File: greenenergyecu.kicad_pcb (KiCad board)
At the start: 4 copper layers, 164 x 118 mm, 103 parts, among them J21 Conn_01x05_Male, J22 USB_B_Mini, M1 Module-power_12and5V-0.3, M2 Module-knock-0.2, M3 Module-vr-discrete-0.5, M4 Module-vr-max9924-0.1, M5 Module-wbo-0.5, M6 Module:mega-mcu100/0.3, M7 Module-can-0.1, M8 Module-motor-driver-0.1, P1 368255-2, Q1 ISL9V3040D3ST, Q2 ISL9V3040D3ST, Q3 ISL9V3040D3ST, Q4 ISL9V3040D3ST, Q5 ISL9V3040D3ST, Q6 ISL9V3040D3ST, Q7 AO3400A, U1 VNLD5160TR-E, U10 BTS6143D, U2 VNLD5160TR-E, U3 VNLD5160TR-E, U4 VNLD5160TR-E, U5 VNLD5160TR-E, U6 VNLD5160TR-E, U7 VNLD5160TR-E, U8 MAX31855KASA

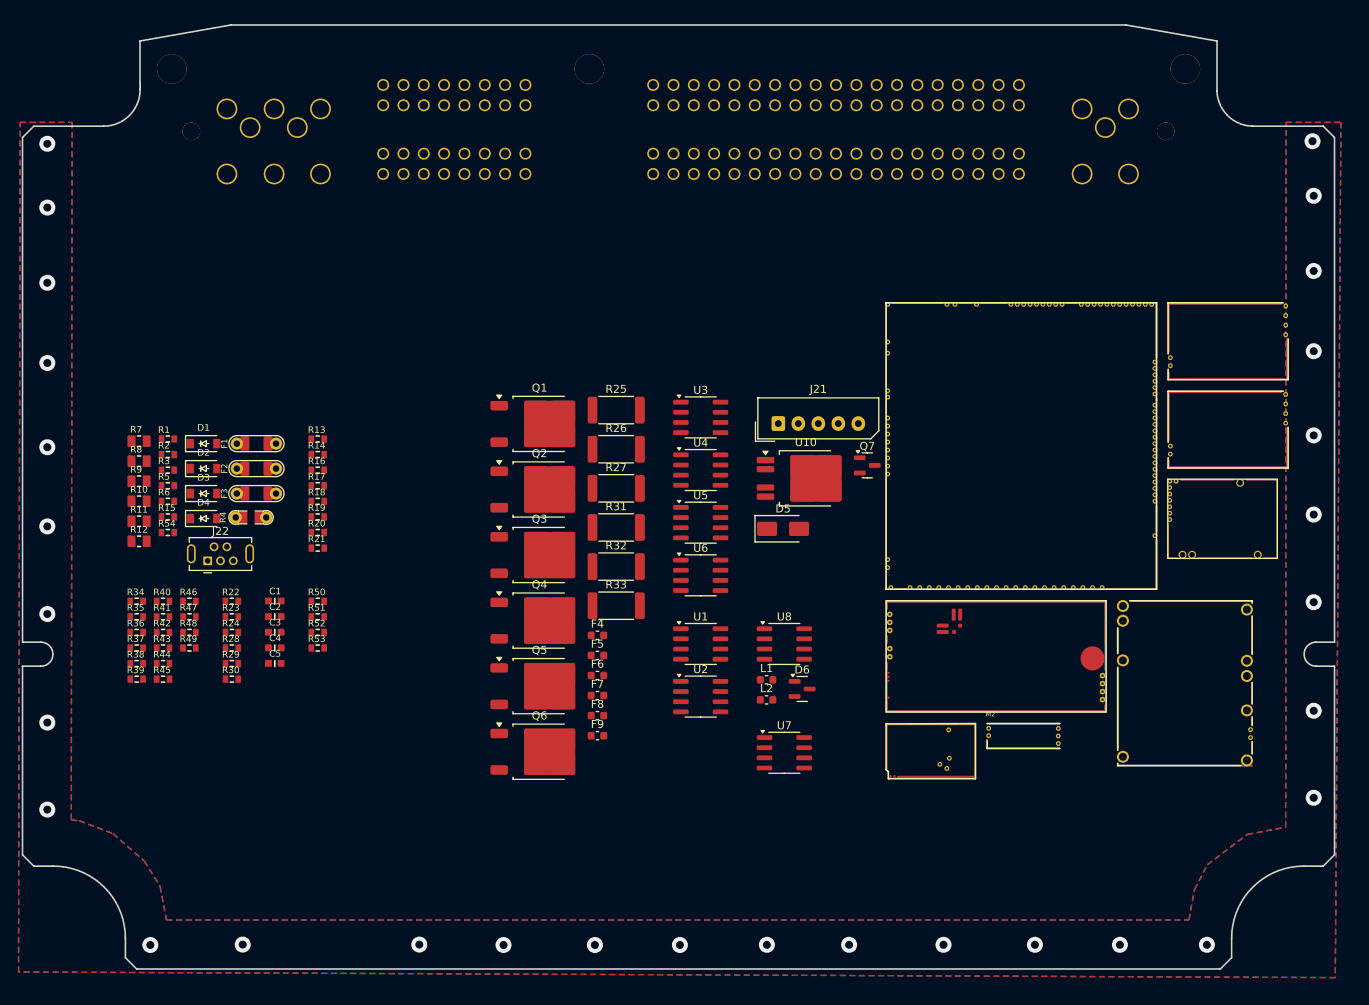
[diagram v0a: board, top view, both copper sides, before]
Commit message: weW
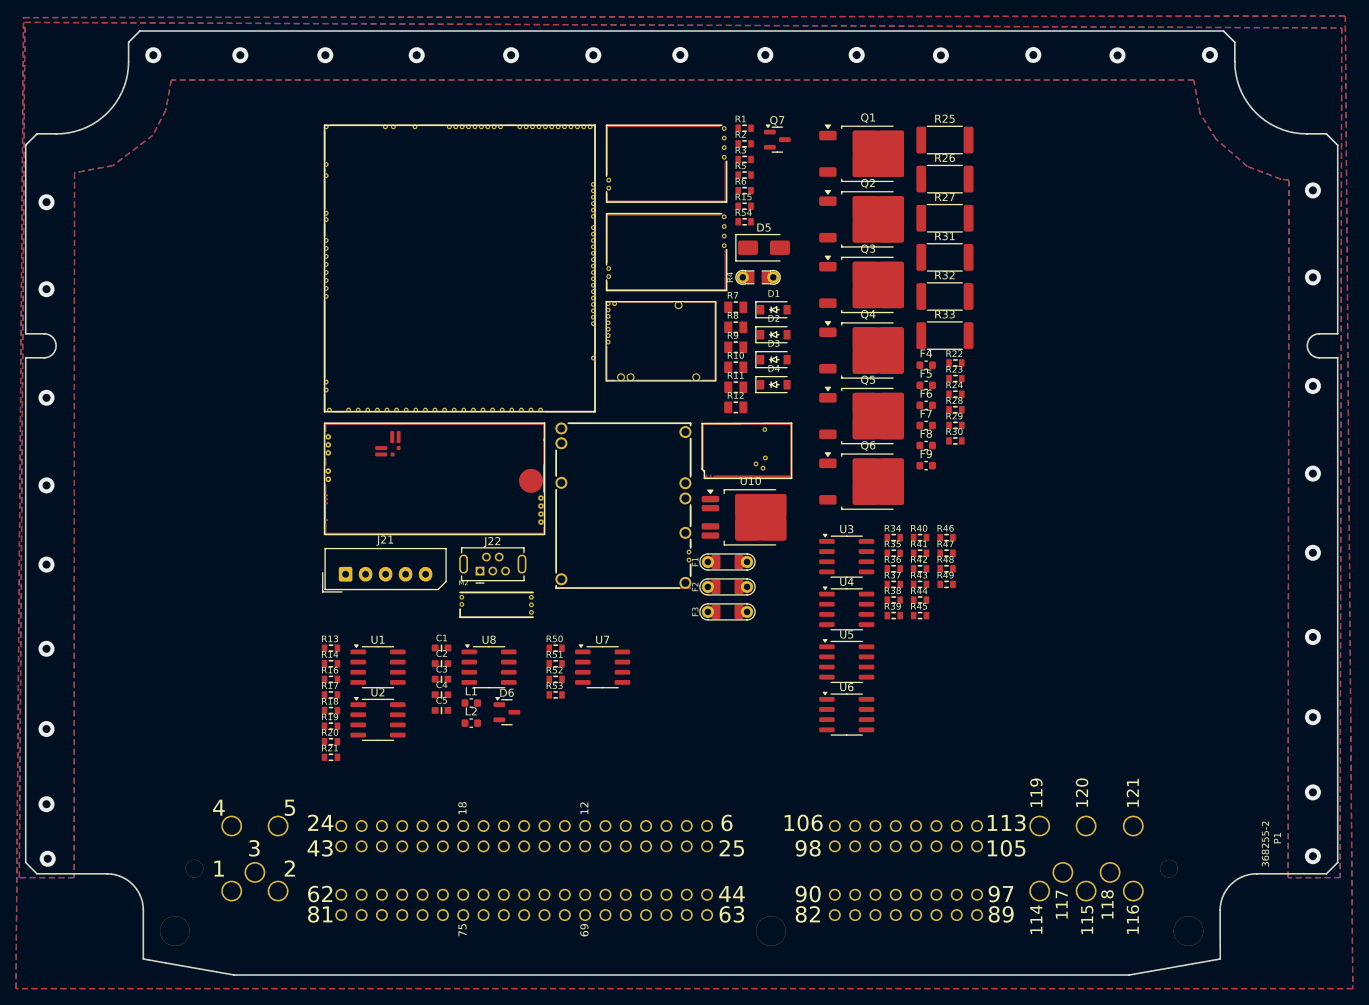
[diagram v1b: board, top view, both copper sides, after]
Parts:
- added G4: DISCLAIMER, rusefi_lib:Off_Road_Disclaimer, B.Cu at (111.8, 0.28)
- P1: footprint 368255-2:368255-2 -> hellen121vag:368255-2
- moved P1 139.4 mm to (60.2, 32.9), turned to 0 degrees
- moved R22 95.2 mm to (161.9, 33.9)
- moved R23 95.2 mm to (161.9, 35.8)
- moved R24 95.2 mm to (161.9, 37.8)
- moved R28 95.2 mm to (161.9, 39.7)
- moved R29 95.2 mm to (161.9, 41.7)
- moved R30 95.2 mm to (161.9, 43.6)
- moved R46 95.0 mm to (160.8, 55.7)
- moved R47 95.0 mm to (160.8, 57.7)
- moved R48 95.0 mm to (160.8, 59.6)
- moved R49 95.0 mm to (160.8, 61.6)
- moved R34 95.0 mm to (154.2, 55.7)
- moved R35 95.0 mm to (154.2, 57.7)
- moved R36 95.0 mm to (154.2, 59.6)
- moved R37 95.0 mm to (154.2, 61.6)
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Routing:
- net PIN2: vias 0 -> 31
- net PIN113: vias 30 -> 0
- added copper zone on B.Cu, net PIN2
- added copper zone on F.Cu, net PIN2
- added copper zone on In1.Cu, net PIN2
- removed copper zone on B.Cu, net PIN113
- removed copper zone on F.Cu, net PIN113
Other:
- outline, holes or cut-outs redrawn
- board text added: "1"
- board text added: "10"
- board text added: "100"
- board text added: "101"
- board text added: "102"
- board text added: "103"
- board text added: "104"
- board text added: "105"
- board text added: "106"
- board text added: "11"
- board text added: "112"
- board text added: "113"
- board text added: "114"
- board text added: "115"
- board text added: "116"
- board text added: "117"
- board text added: "118"
- board text added: "119"
- board text added: "12"
- board text added: "120"
- board text added: "121"
- board text added: "13"
- board text added: "14"
- board text added: "15"
- board text added: "16"
- board text added: "17"
- board text added: "18"
- board text added: "19"
- board text added: "2"
- board text added: "20"
- board text added: "21"
- board text added: "22"
- board text added: "23"
- board text added: "24"
- board text added: "25"
- board text added: "26"
- board text added: "27"
- board text added: "28"
- board text added: "29"
- board text added: "3"
- board text added: "30"
- board text added: "31"
- board text added: "32"
- board text added: "33"
- board text added: "34"
- board text added: "35"
- board text added: "36"
- board text added: "37"
- board text added: "38"
- board text added: "39"
- board text added: "4"
- board text added: "40"
- board text added: "41"
- board text added: "42"
- board text added: "43"
- board text added: "44"
- board text added: "45"
- board text added: "46"
- board text added: "47"
- board text added: "48"
- board text added: "49"
- board text added: "5"
- board text added: "50"
- board text added: "51"
- board text added: "52"
- board text added: "53"
- board text added: "54"
- board text added: "55"
- board text added: "56"
- board text added: "57"
- board text added: "58"
- board text added: "59"
- board text added: "6"
- board text added: "60"
- board text added: "61"
- board text added: "62"
- board text added: "63"
- board text added: "64"
- board text added: "65"
- board text added: "66"
- board text added: "67"
- board text added: "68"
- board text added: "69"
- board text added: "7"
- board text added: "70"
- board text added: "71"
- board text added: "72"
- board text added: "73"
- board text added: "74"
- board text added: "75"
- board text added: "76"
- board text added: "77"
- board text added: "78"
- board text added: "79"
- board text added: "8"
- board text added: "80"
- board text added: "81"
- board text added: "82"
- board text added: "83"
- board text added: "84"
- board text added: "85"
- board text added: "86"
- board text added: "87"
- board text added: "88"
- board text added: "89"
- board text added: "9"
- board text added: "90"
- board text added: "91"
- board text added: "92"
- board text added: "93"
- board text added: "94"
- board text added: "95"
- board text added: "96"
- board text added: "97"
- board text added: "98"
- board text added: "99"

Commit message: weW
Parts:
- removed G4: DISCLAIMER, rusefi_lib:Off_Road_Disclaimer
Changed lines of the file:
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@@
 		)
-	)
-	(footprint "rusefi_lib:Off_Road_Disclaimer"
-		(locked yes)
-		(layer "B.Cu")
-		(at 111.75 0.275 180)
-		(property "Reference" "G4"
-			(at 0 5.715 0)
-			(layer "B.SilkS")
-			(hide yes)
-			(effects
-				(font
-					(size 1.524 1.524)
-					(thickness 0.3048)
-				)
-				(justify mirror)
-			)
-		)
-		(property "Value" "DISCLAIMER"
-			(at 0 8.255 0)
-			(layer "B.SilkS")
-			(hide yes)
-			(effects
-				(font
-					(size 1.524 1.524)
-					(thickness 0.3048)
-				)
-				(justify mirror)
-			)
-		)
-		(property "Footprint" ""
-			(at 0 0 180)
-			(layer "F.Fab")
-			(hide yes)
-			(effects
-				(font
-					(size 1.27 1.27)
-					(thickness 0.15)
-				)
-			)
-		)
-		(property "Datasheet" ""
-			(at 0 0 180)
-			(layer "F.Fab")
-			(hide yes)
-			(effects
-				(font
-					(size 1.27 1.27)
-					(thickness 0.15)
-				)
-			)
-		)
-		(property "Description" ""
-			(at 0 0 180)
-			(layer "F.Fab")
-			(hide yes)
-			(effects
-				(font
-					(size 1.27 1.27)
-					(thickness 0.15)
-				)
-			)
-		)
-		(sheetfile "hellen121vag.kicad_sch")
-		(attr through_hole)
 	)
 	(gr_line
@@
 		(min_thickness 0.254)
 		(filled_areas_thickness no)
-		(fill
+		(fill yes
 			(thermal_gap 0.508)
 			(thermal_bridge_width 0.508)
@@
 		(min_thickness 0.2)
 		(filled_areas_thickness no)
-		(fill
+		(fill yes
 			(thermal_gap 0.2)
 			(thermal_bridge_width 0.5)
@@
 		(min_thickness 0.254)
 		(filled_areas_thickness no)
-		(fill
+		(fill yes
 			(thermal_gap 0.508)
 			(thermal_bridge_width 0.508)
@@
 		(min_thickness 0.2)
 		(filled_areas_thickness no)
-		(fill
+		(fill yes
 			(thermal_gap 0.2)
 			(thermal_bridge_width 0.5)
@@
 		(min_thickness 0.2)
 		(filled_areas_thickness no)
-		(fill
+		(fill yes
 			(thermal_gap 0.2)
 			(thermal_bridge_width 0.5)
@@
 		(min_thickness 0.2)
 		(filled_areas_thickness no)
-		(fill
+		(fill yes
 			(thermal_gap 0.2)
 			(thermal_bridge_width 0.5)
@@
 		(min_thickness 0.2)
 		(filled_areas_thickness no)
-		(fill
+		(fill yes
 			(thermal_gap 0.2)
 			(thermal_bridge_width 0.5)
@@
 		(min_thickness 0.2)
 		(filled_areas_thickness no)
-		(fill
+		(fill yes
 			(thermal_gap 0.2)
 			(thermal_bridge_width 0.5)
